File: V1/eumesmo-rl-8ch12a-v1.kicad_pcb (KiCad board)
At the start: 2 copper layers, 98 x 67.8 mm, 48 parts, among them J1 250-202, J2 250-204, J3 250-204, J4 DB142V-5.08-4P, J5 DB142V-5.08-4P, J6 DB142V-5.08-4P, J7 DB142V-5.08-4P, K1 G5PZ-1A, K2 G5PZ-1A, K3 G5PZ-1A, K4 G5PZ-1A, K5 G5PZ-1A, K6 G5PZ-1A, K7 G5PZ-1A, K8 G5PZ-1A

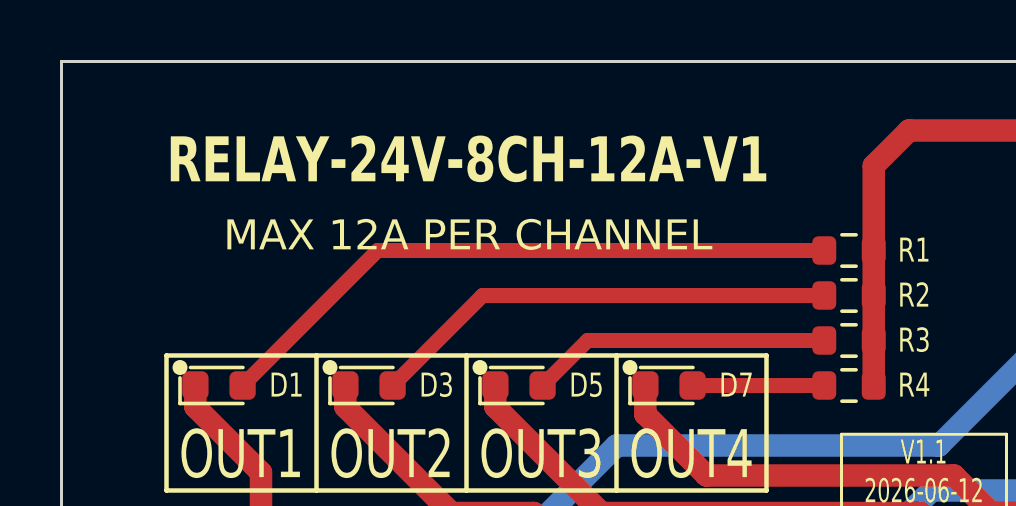
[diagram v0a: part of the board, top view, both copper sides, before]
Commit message: Adjusted version numbers.
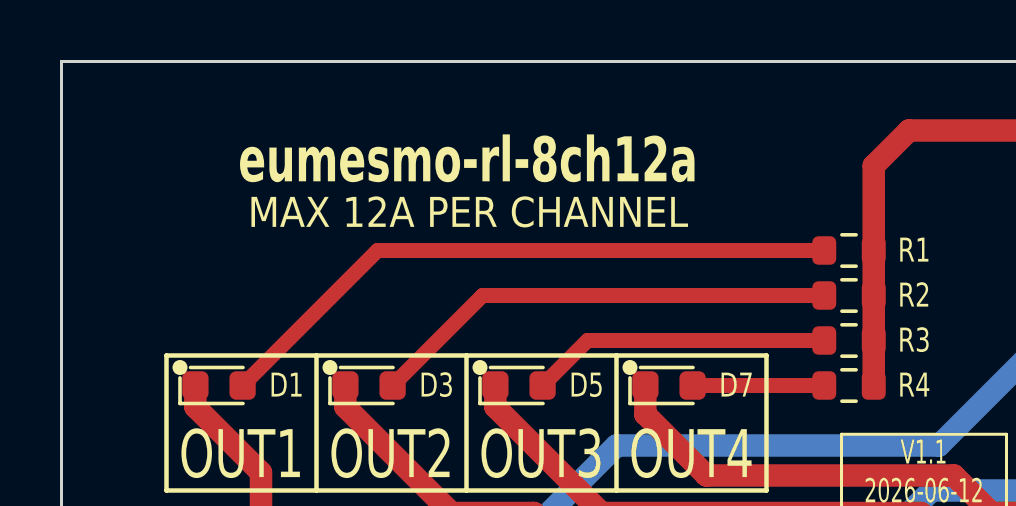
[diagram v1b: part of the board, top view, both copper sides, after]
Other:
- board text added: "eumesmo-rl-8ch12a"
- board text removed: "RELAY-24V-8CH-12A-V1"
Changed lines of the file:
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@@
 	(paper "A4")
 	(title_block
-		(title "8x 24V 12A Relay Module")
-		(date "2026-06-12")
-		(rev "V1.1")
+		(title "eumesmo 8x 24V 12A NO Relay Module")
+		(date "2026-06-13")
+		(rev "V1.2")
 	)
 	(layers
@@
 	)
 	(gr_text "MAX 12A PER CHANNEL"
-		(at 138.55 68 0)
+		(at 138.55 67.25 0)
 		(layer "F.SilkS")
 		(effects
 			(font
-				(size 1 1)
+				(size 1 0.9)
 				(thickness 0.15)
 			)
@@
 		)
 	)
-	(gr_text "RELAY-24V-8CH-12A-V1"
+	(gr_text "eumesmo-rl-8ch12a"
 		(at 138.55 65.5 0)
 		(layer "F.SilkS")
 		(effects
 			(font
-				(size 1.5 1.1)
-				(thickness 0.25)
+				(size 1.5 1)
+				(thickness 0.2)
 				(bold yes)
 			)
